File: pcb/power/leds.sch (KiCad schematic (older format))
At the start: 26 parts, among them U4 LM324QT

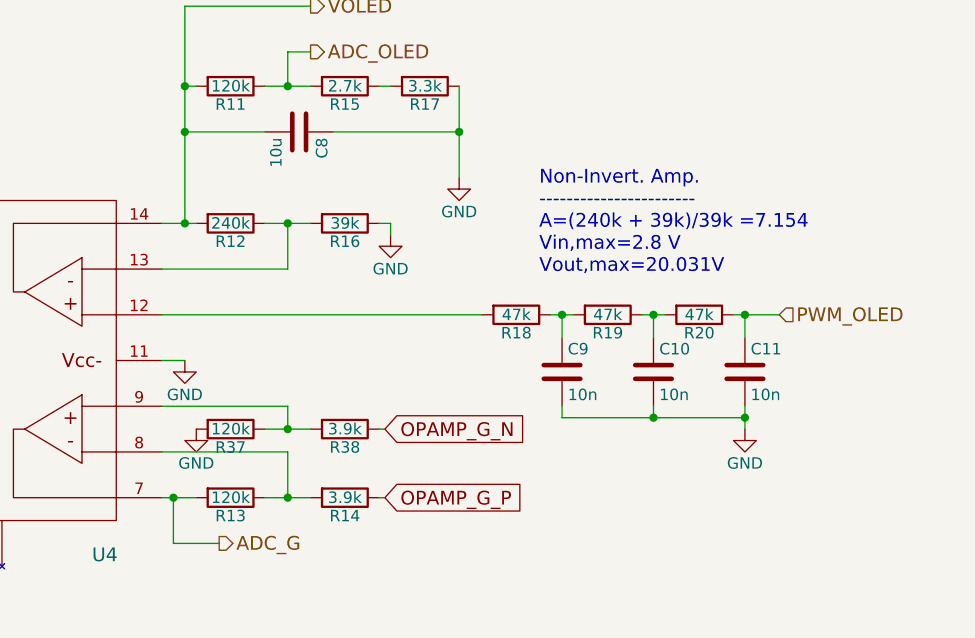
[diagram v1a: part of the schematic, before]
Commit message: Fixed the board. This is rev 2.
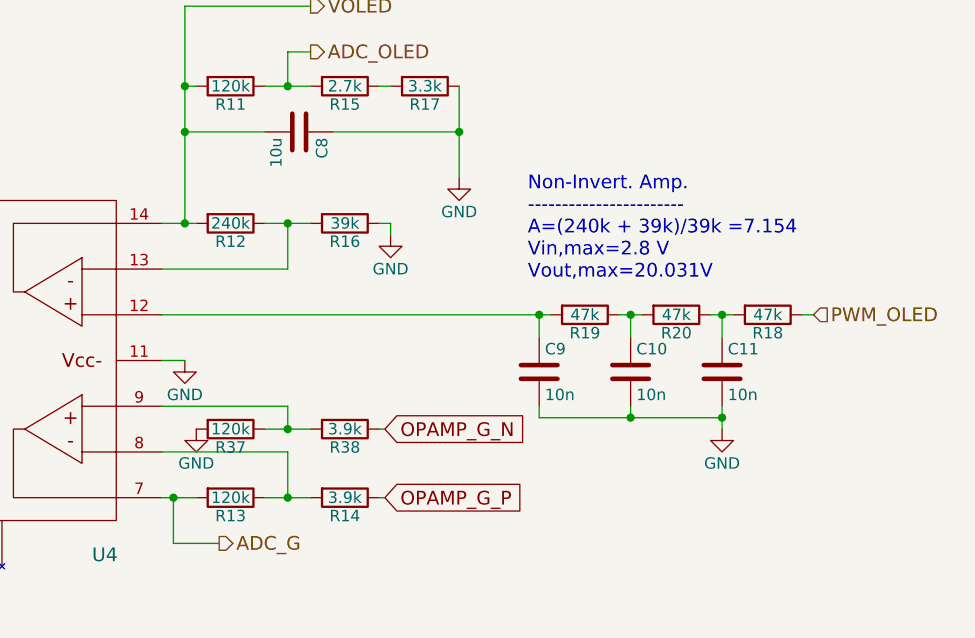
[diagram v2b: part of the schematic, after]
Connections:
- net PWM_OLED: now also R18.1; no longer C11.1, R20.1
- net at U4.12 (P_4): now also C9.1, R19.2; no longer R18.2
- new net: C11.1, R18.2, R20.1
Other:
- moved on the sheet: C10, C11, C9, R18, R19, R20
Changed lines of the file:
@@
 L R R18
 U 1 1 58430FD2
-P 9250 3475
-F 0 "R18" V 9330 3475 50  0000 C CNN
-F 1 "47k" V 9250 3475 50  0000 C CNN
-F 2 "Additional:R_0603_HandSoldering_Same_As_C" V 9180 3475 50  0001 C CNN
-F 3 "http://www.yageo.com.tw/exep/pages/download/literatures/PYu-R_INT-thick_7.pdf" H 9250 3475 50  0001 C CNN
-F 4 "311-47.0KHRCT-ND" V 9250 3475 60  0001 C CNN "Digikey"
-	1    9250 3475
+P 10350 3475
+F 0 "R18" V 10430 3475 50  0000 C CNN
+F 1 "47k" V 10350 3475 50  0000 C CNN
+F 2 "Additional:R_0603_HandSoldering_Same_As_C" V 10280 3475 50  0001 C CNN
+F 3 "http://www.yageo.com.tw/exep/pages/download/literatures/PYu-R_INT-thick_7.pdf" H 10350 3475 50  0001 C CNN
+F 4 "311-47.0KHRCT-ND" V 10350 3475 60  0001 C CNN "Digikey"
+	1    10350 3475
 	0    1    1    0
 $EndComp
@@
 L C C9
 U 1 1 58430FDA
-P 9450 3725
-F 0 "C9" H 9475 3825 50  0000 L CNN
-F 1 "10n" H 9475 3625 50  0000 L CNN
-F 2 "Capacitors_SMD:C_0603_HandSoldering" H 9488 3575 50  0001 C CNN
-F 3 "http://www.yageo.com/documents/recent/UPY-GPHC_X7R_6.3V-to-50V_15.pdf" H 9450 3725 50  0001 C CNN
-F 4 "311-1085-1-ND" H 9450 3725 60  0001 C CNN "Digikey"
-	1    9450 3725
+P 9350 3725
+F 0 "C9" H 9375 3825 50  0000 L CNN
+F 1 "10n" H 9375 3625 50  0000 L CNN
+F 2 "Capacitors_SMD:C_0603_HandSoldering" H 9388 3575 50  0001 C CNN
+F 3 "http://www.yageo.com/documents/recent/UPY-GPHC_X7R_6.3V-to-50V_15.pdf" H 9350 3725 50  0001 C CNN
+F 4 "311-1085-1-ND" H 9350 3725 60  0001 C CNN "Digikey"
+	1    9350 3725
 	1    0    0    -1
 $EndComp
@@
 L GND #PWR018
 U 1 1 58430FE1
-P 10250 3975
-F 0 "#PWR018" H 10250 3725 50  0001 C CNN
-F 1 "GND" H 10250 3825 50  0000 C CNN
-F 2 "" H 10250 3975 50  0000 C CNN
-F 3 "" H 10250 3975 50  0000 C CNN
-	1    10250 3975
+P 10150 3975
+F 0 "#PWR018" H 10150 3725 50  0001 C CNN
+F 1 "GND" H 10150 3825 50  0000 C CNN
+F 2 "" H 10150 3975 50  0000 C CNN
+F 3 "" H 10150 3975 50  0000 C CNN
+	1    10150 3975
 	1    0    0    -1
 $EndComp
@@
 L R R19
 U 1 1 58431010
-P 9650 3475
-F 0 "R19" V 9730 3475 50  0000 C CNN
-F 1 "47k" V 9650 3475 50  0000 C CNN
-F 2 "Additional:R_0603_HandSoldering_Same_As_C" V 9580 3475 50  0001 C CNN
-F 3 "http://www.yageo.com.tw/exep/pages/download/literatures/PYu-R_INT-thick_7.pdf" H 9650 3475 50  0001 C CNN
-F 4 "311-47.0KHRCT-ND" V 9650 3475 60  0001 C CNN "Digikey"
-	1    9650 3475
+P 9550 3475
+F 0 "R19" V 9630 3475 50  0000 C CNN
+F 1 "47k" V 9550 3475 50  0000 C CNN
+F 2 "Additional:R_0603_HandSoldering_Same_As_C" V 9480 3475 50  0001 C CNN
+F 3 "http://www.yageo.com.tw/exep/pages/download/literatures/PYu-R_INT-thick_7.pdf" H 9550 3475 50  0001 C CNN
+F 4 "311-47.0KHRCT-ND" V 9550 3475 60  0001 C CNN "Digikey"
+	1    9550 3475
 	0    1    1    0
 $EndComp
@@
 L R R20
 U 1 1 58431018
-P 10050 3475
-F 0 "R20" V 10130 3475 50  0000 C CNN
-F 1 "47k" V 10050 3475 50  0000 C CNN
-F 2 "Additional:R_0603_HandSoldering_Same_As_C" V 9980 3475 50  0001 C CNN
-F 3 "http://www.yageo.com.tw/exep/pages/download/literatures/PYu-R_INT-thick_7.pdf" H 10050 3475 50  0001 C CNN
-F 4 "311-47.0KHRCT-ND" V 10050 3475 60  0001 C CNN "Digikey"
-	1    10050 3475
+P 9950 3475
+F 0 "R20" V 10030 3475 50  0000 C CNN
+F 1 "47k" V 9950 3475 50  0000 C CNN
+F 2 "Additional:R_0603_HandSoldering_Same_As_C" V 9880 3475 50  0001 C CNN
+F 3 "http://www.yageo.com.tw/exep/pages/download/literatures/PYu-R_INT-thick_7.pdf" H 9950 3475 50  0001 C CNN
+F 4 "311-47.0KHRCT-ND" V 9950 3475 60  0001 C CNN "Digikey"
+	1    9950 3475
 	0    1    1    0
 $EndComp
@@
 L C C10
 U 1 1 58431020
-P 9850 3725
-F 0 "C10" H 9875 3825 50  0000 L CNN
-F 1 "10n" H 9875 3625 50  0000 L CNN
-F 2 "Capacitors_SMD:C_0603_HandSoldering" H 9888 3575 50  0001 C CNN
-F 3 "http://www.yageo.com/documents/recent/UPY-GPHC_X7R_6.3V-to-50V_15.pdf" H 9850 3725 50  0001 C CNN
-F 4 "311-1085-1-ND" H 9850 3725 60  0001 C CNN "Digikey"
-	1    9850 3725
+P 9750 3725
+F 0 "C10" H 9775 3825 50  0000 L CNN
+F 1 "10n" H 9775 3625 50  0000 L CNN
+F 2 "Capacitors_SMD:C_0603_HandSoldering" H 9788 3575 50  0001 C CNN
+F 3 "http://www.yageo.com/documents/recent/UPY-GPHC_X7R_6.3V-to-50V_15.pdf" H 9750 3725 50  0001 C CNN
+F 4 "311-1085-1-ND" H 9750 3725 60  0001 C CNN "Digikey"
+	1    9750 3725
 	1    0    0    -1
 $EndComp
@@
 L C C11
 U 1 1 58431029
-P 10250 3725
-F 0 "C11" H 10275 3825 50  0000 L CNN
-F 1 "10n" H 10275 3625 50  0000 L CNN
-F 2 "Capacitors_SMD:C_0603_HandSoldering" H 10288 3575 50  0001 C CNN
-F 3 "http://www.yageo.com/documents/recent/UPY-GPHC_X7R_6.3V-to-50V_15.pdf" H 10250 3725 50  0001 C CNN
-F 4 "311-1085-1-ND" H 10250 3725 60  0001 C CNN "Digikey"
-	1    10250 3725
+P 10150 3725
+F 0 "C11" H 10175 3825 50  0000 L CNN
+F 1 "10n" H 10175 3625 50  0000 L CNN
+F 2 "Capacitors_SMD:C_0603_HandSoldering" H 10188 3575 50  0001 C CNN
+F 3 "http://www.yageo.com/documents/recent/UPY-GPHC_X7R_6.3V-to-50V_15.pdf" H 10150 3725 50  0001 C CNN
+F 4 "311-1085-1-ND" H 10150 3725 60  0001 C CNN "Digikey"
+	1    10150 3725
 	1    0    0    -1
 $EndComp
@@
 	1    0    0    -1
 $EndComp
-Text Notes 9350 3300 0    60   ~ 0
+Text Notes 9300 3325 0    60   ~ 0
 Non-Invert. Amp.\n-----------------------\nA=(240k + 39k)/39k =7.154\nVin,max=2.8 V\nVout,max=20.031V
 Text Notes 4750 5075 0    60   ~ 0
@@
 Text HLabel 7950 4475 2    60   Output ~ 0
 ADC_G
-Text HLabel 10400 3475 2    60   Input ~ 0
+Text HLabel 10550 3475 2    60   Input ~ 0
 PWM_OLED
 Text HLabel 8350 2325 2    60   Output ~ 0
@@
 $EndComp
 Wire Wire Line
-	9400 3475 9500 3475
-Wire Wire Line
-	9800 3475 9900 3475
-Wire Wire Line
-	9450 3925 10250 3925
-Wire Wire Line
-	9450 3925 9450 3875
-Connection ~ 10250 3925
-Wire Wire Line
-	9850 3875 9850 3925
-Connection ~ 9850 3925
-Wire Wire Line
-	9450 3575 9450 3475
-Connection ~ 9450 3475
-Wire Wire Line
-	9850 3575 9850 3475
-Connection ~ 9850 3475
-Wire Wire Line
-	10250 3875 10250 3975
-Wire Wire Line
-	10250 3575 10250 3475
-Wire Wire Line
-	10200 3475 10400 3475
-Connection ~ 10250 3475
+	9700 3475 9800 3475
+Wire Wire Line
+	9350 3925 10150 3925
+Wire Wire Line
+	9350 3925 9350 3875
+Connection ~ 10150 3925
+Wire Wire Line
+	9750 3875 9750 3925
+Connection ~ 9750 3925
+Wire Wire Line
+	9750 3575 9750 3475
+Connection ~ 9750 3475
+Wire Wire Line
+	10150 3875 10150 3975
 Wire Wire Line
 	7700 3275 8250 3275
@@
 Wire Wire Line
 	7700 4075 8250 4075
-Wire Wire Line
-	7700 3475 9100 3475
 Connection ~ 5700 4275
 Wire Wire Line
@@
 Wire Wire Line
 	6300 3200 6300 3275
+Wire Wire Line
+	7700 3475 9400 3475
+Wire Wire Line
+	9350 3575 9350 3475
+Connection ~ 9350 3475
+Wire Wire Line
+	10100 3475 10200 3475
+Wire Wire Line
+	10150 3475 10150 3575
+Connection ~ 10150 3475
+Wire Wire Line
+	10500 3475 10550 3475
 $EndSCHEMATC
